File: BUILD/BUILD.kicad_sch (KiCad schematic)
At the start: 18 parts, among them J1-INPUT1 AudioJack3, SW1 SW_Push, SW2 SW_Push, SW3 SW_DIP_x04, SW4 SW_Push, U2 ADC081C021CIMM

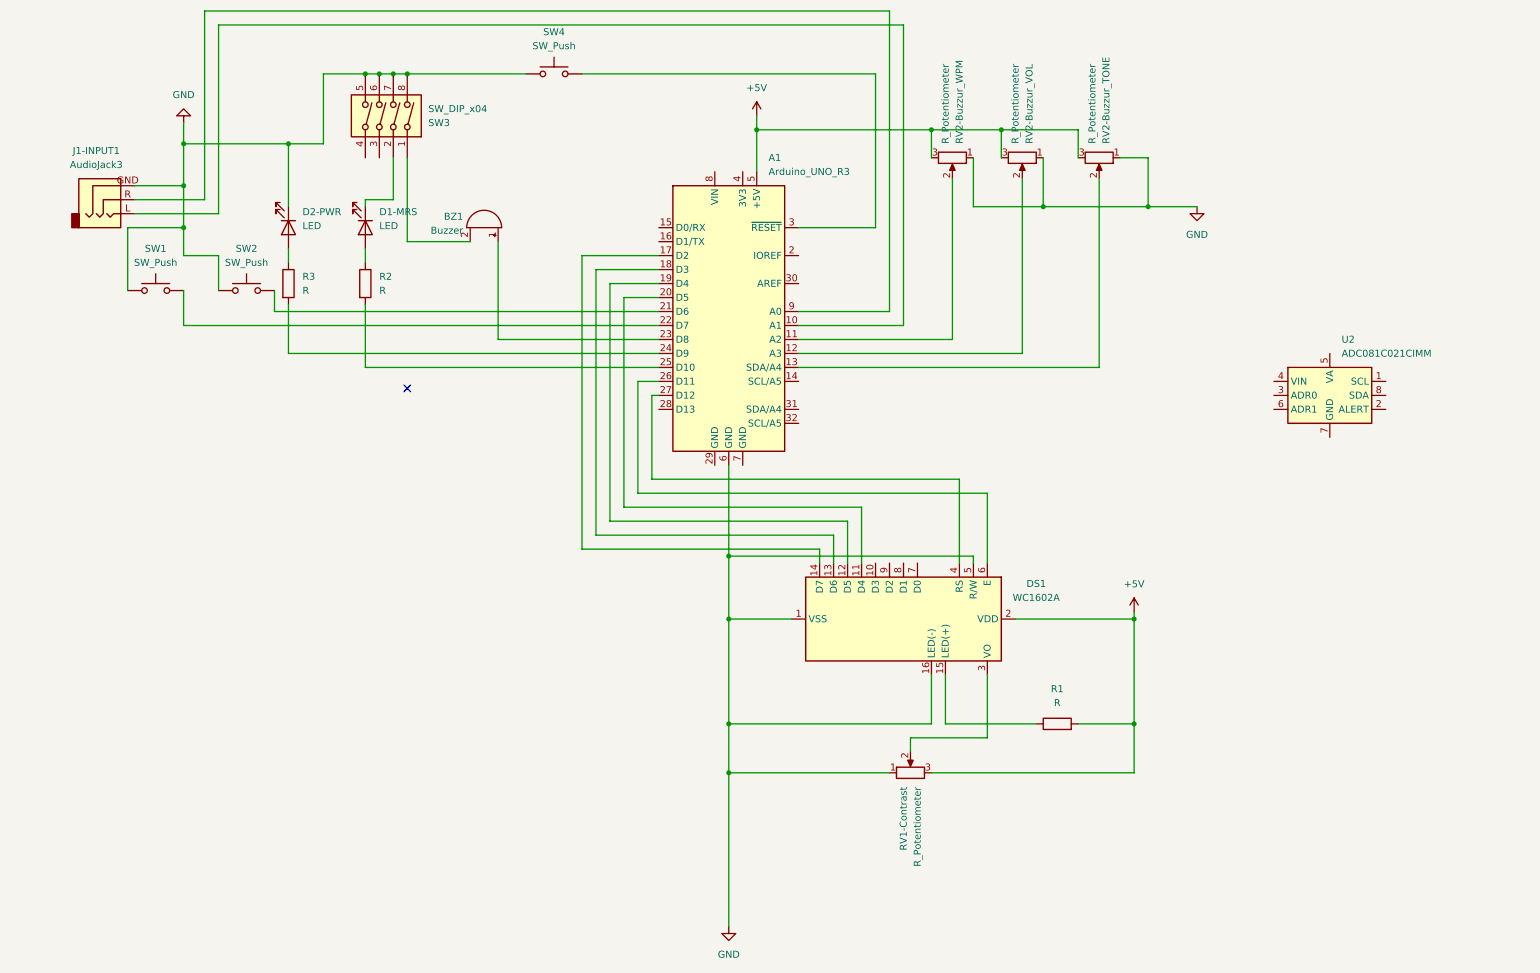
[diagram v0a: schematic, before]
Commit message: 2025-06-19-01
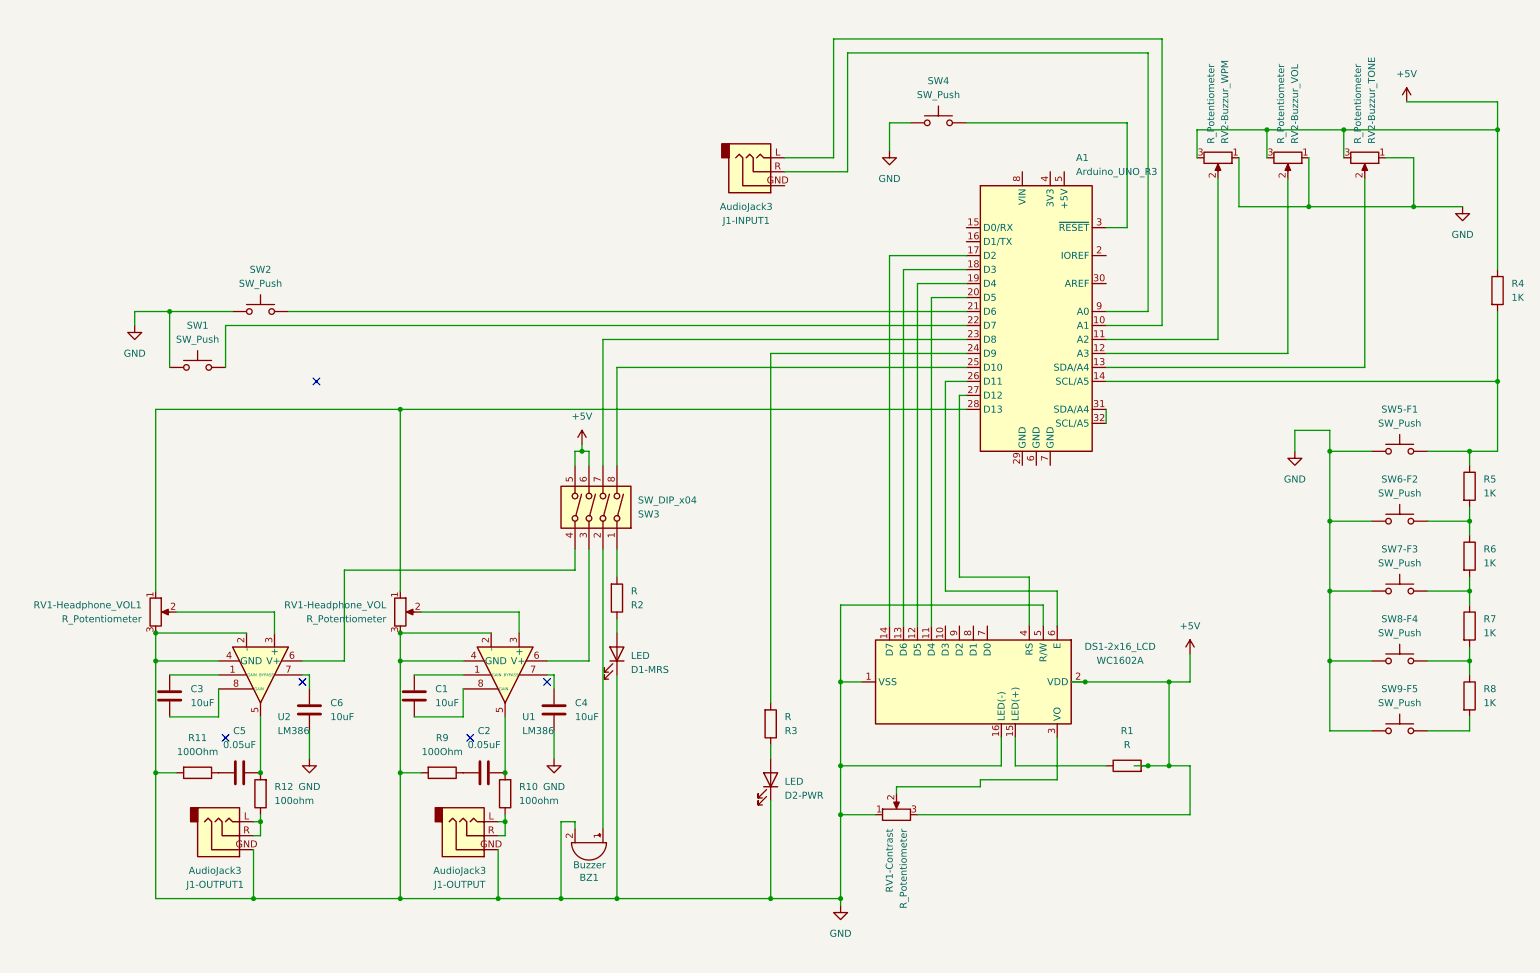
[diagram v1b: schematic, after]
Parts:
- removed U2: ADC081C021CIMM, Package_SO:MSOP-8_3x3mm_P0.65mm, symbol Analog_ADC:ADC081C021CIMM
- added C1, C3, C4, C6: 10uF, symbol Device:C
- added C2, C5: 0.05uF, symbol Device:C
- added J1-OUTPUT, J1-OUTPUT1: AudioJack3, symbol Connector_Audio:AudioJack3
- added R10, R12: 100ohm, symbol Device:R
- added R11, R9: 100Ohm, symbol Device:R
- added R4, R5, R6, R7, R8: 1K, symbol Device:R
- added RV1-Headphone_VOL, RV1-Headphone_VOL1: R_Potentiometer, symbol Device:R_Potentiometer
- added SW5-F1, SW6-F2, SW7-F3, SW8-F4, SW9-F5: SW_Push, symbol Switch:SW_Push
- added U1, U2: LM386, symbol Amplifier_Audio:LM386
- renumbered DS1 to DS1-2x16_LCD
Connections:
- net +5V: now also SW3.5, SW3.6, R4.1; no longer A1.5 (+5V)
- net GND: now also BZ1.2 (-), D1-MRS.1 (K), C4.2, C6.2, J1-OUTPUT.GND, J1-OUTPUT1.GND, R11.2, R9.2, RV1-Headphone_VOL.3, RV1-Headphone_VOL1.3, SW5-F1.1, SW6-F2.1, SW7-F3.1, SW8-F4.1, SW9-F5.1, U1.2 (-), U1.4 (GND), U2.2 (-), U2.4 (GND); no longer A1.6 (GND), J1-INPUT1.GND, SW3.5, SW3.6, SW3.7, SW3.8
- net at A1.14 (SCL/A5): now also R4.2, R5.1, SW5-F1.2
- net at A1.23 (D8): now also SW3.7; no longer BZ1.1 (+)
- net at A1.25 (D10): now also SW3.8; no longer R2.2
- net at A1.28 (D13): now also RV1-Headphone_VOL.1, RV1-Headphone_VOL1.1
- net at A1.31 (SDA/A4): now also A1.32 (SCL/A5)
- net at SW3.2: now also BZ1.1 (+); no longer D1-MRS.1 (K)
- net at SW3.1: now also R2.2; no longer BZ1.2 (-)
- net at SW3.3: now also U1.6 (V+)
- net at SW3.4: now also U2.6 (V+)
- new net: RV1-Headphone_VOL.2, U1.3 (+)
- new net: C2.1, R10.2, U1.5
- new net: C2.2, R9.1
- new net: J1-OUTPUT.L, J1-OUTPUT.R, R10.1
- new net: R5.2, R6.1, SW6-F2.2
- new net: J1-OUTPUT1.L, J1-OUTPUT1.R, R12.1
- new net: C5.1, R12.2, U2.5
- new net: R6.2, R7.1, SW7-F3.2
- new net: R8.2, SW9-F5.2
- new net: C1.1, U1.1 (GAIN)
- new net: C4.1, U1.7 (BYPASS)
- new net: C1.2, U1.8 (GAIN)
- new net: C5.2, R11.1
- new net: R7.2, R8.1, SW8-F4.2
- new net: C6.1, U2.7 (BYPASS)
- new net: C3.1, U2.1 (GAIN)
- new net: C3.2, U2.8 (GAIN)
- new net: RV1-Headphone_VOL1.2, U2.3 (+)
- no-connect marks 1 -> 5
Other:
- moved on the sheet: A1, BZ1, D1-MRS, D2-PWR, DS1-2x16_LCD, J1-INPUT1, R1, R2, R3, RV1-Contrast, RV2-Buzzur_TONE, RV2-Buzzur_VOL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
